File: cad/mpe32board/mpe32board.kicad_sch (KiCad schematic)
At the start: 2 parts, among them J1 Conn_ST_STDC14, U2 STM32H743VIHx

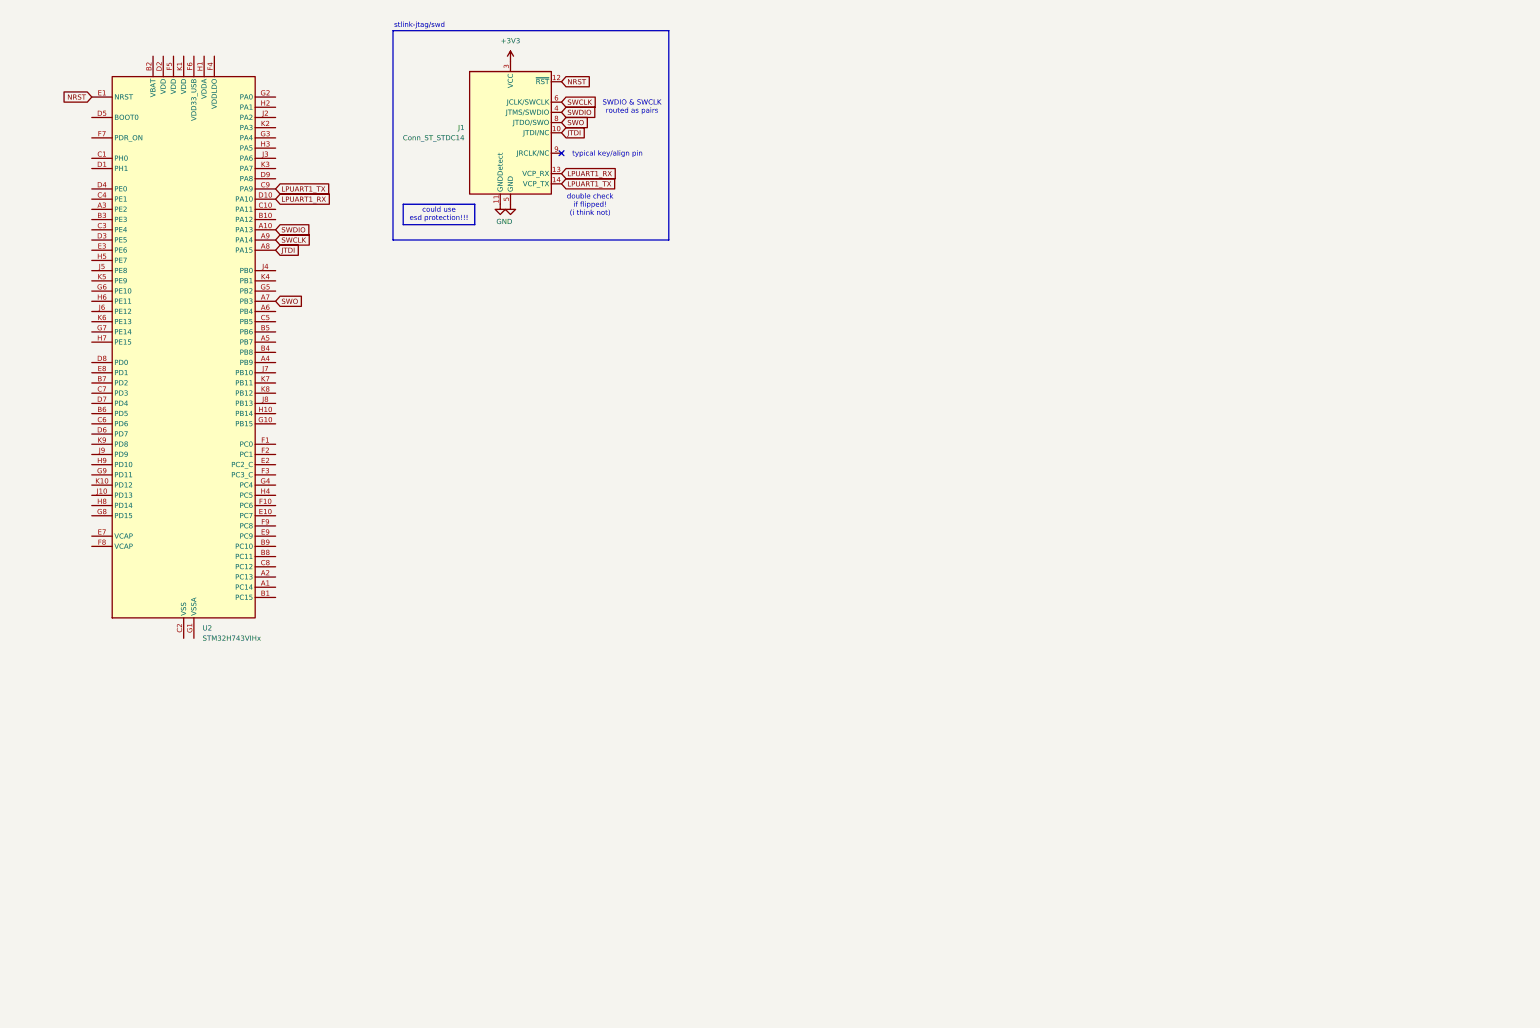
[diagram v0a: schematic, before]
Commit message: more pcb additions + research
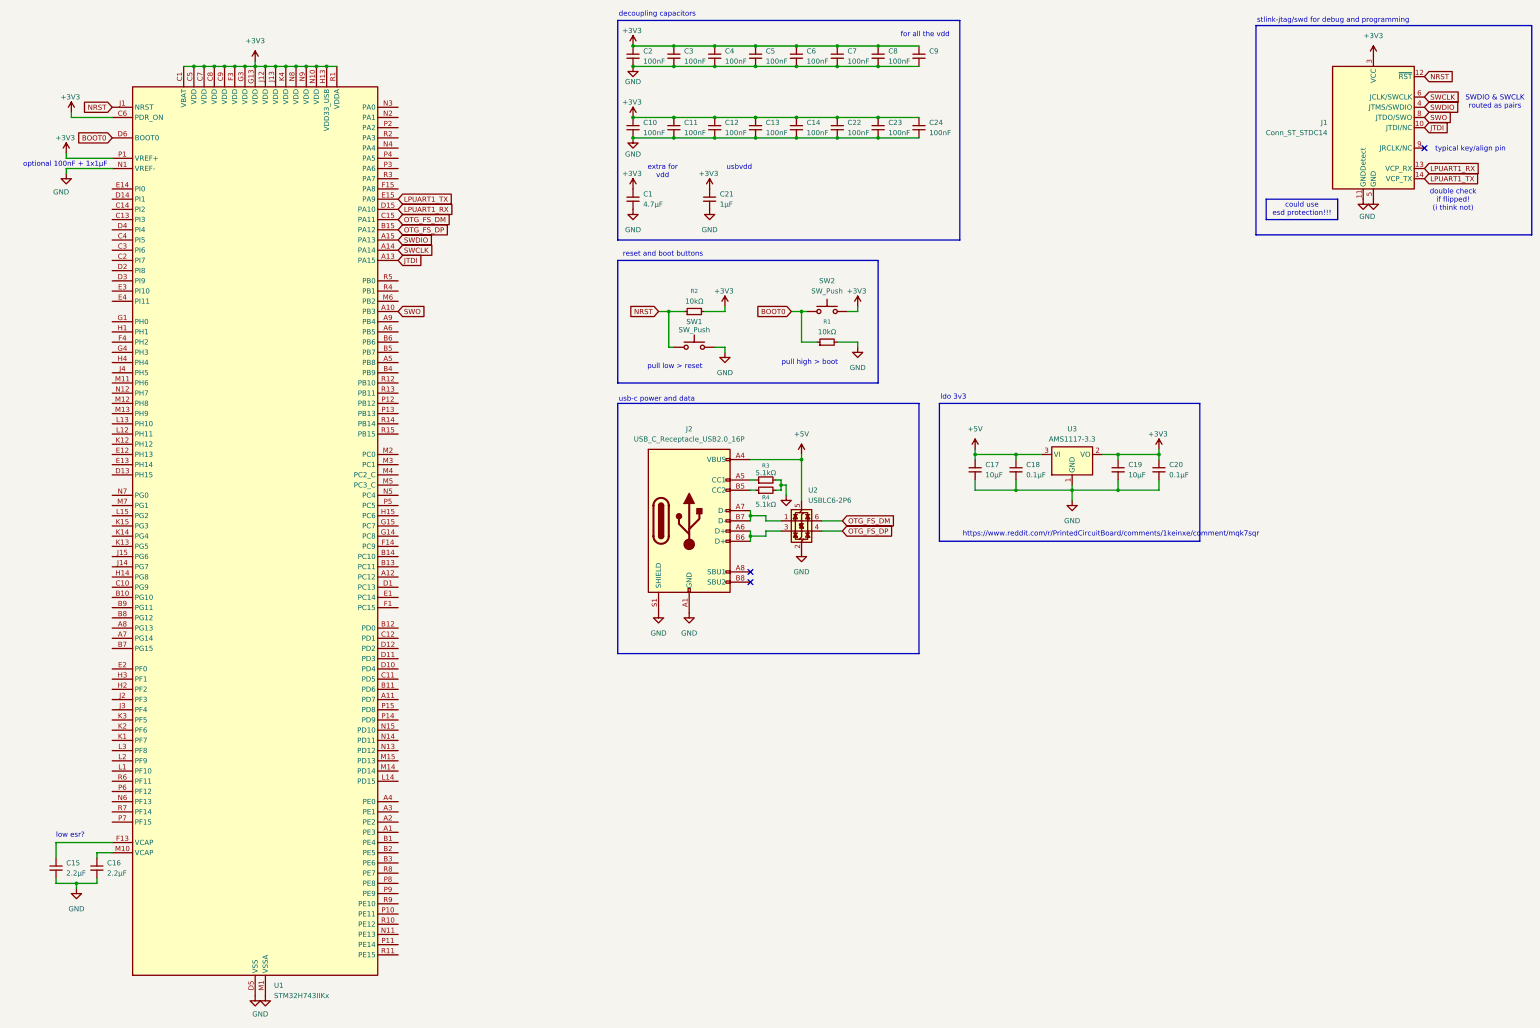
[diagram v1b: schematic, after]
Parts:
- removed U2: STM32H743VIHx, Package_BGA:TFBGA-100_8x8mm_Layout10x10_P0.8mm, symbol MCU_ST_STM32H7:STM32H743VIHx
- added C1: 4.7μF, symbol Device:C_Small
- added C10, C11, C12, C13, C14, C2, C22, C23, C24, C3, C4, C5, C6, C7, C8, C9: 100nF, symbol Device:C_Small
- added C15, C16: 2.2μF, symbol Device:C_Small
- added C17, C19: 10μF, symbol Device:C_Small
- added C18, C20: 0.1μF, symbol Device:C_Small
- added C21: 1μF, symbol Device:C_Small
- added J2: USB_C_Receptacle_USB2.0_16P, symbol Connector:USB_C_Receptacle_USB2.0_16P
- added R1, R2: 10kΩ, symbol Device:R_Small
- added R3, R4: 5.1kΩ, symbol Device:R_Small
- added SW1, SW2: SW_Push, symbol Switch:SW_Push
- added U1: STM32H743IIKx, Package_BGA:UFBGA-201_10x10mm_Layout15x15_P0.65mm, symbol MCU_ST_STM32H7:STM32H743IIKx
- added U2: USBLC6-2P6, Package_TO_SOT_SMD:SOT-666, symbol Power_Protection:USBLC6-2P6
- added U3: AMS1117-3.3, Package_TO_SOT_SMD:SOT-223-3_TabPin2, symbol Regulator_Linear:AMS1117-3.3
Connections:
- net +3V3: now also C1.1, C10.1, C11.1, C12.1, C13.1, C14.1, C19.1, C2.1, C20.1, C21.1, C22.1, C23.1, C24.1, C3.1, C4.1, C5.1, C6.1, C7.1, C8.1, C9.1, R2.2, SW2.2, U1.C1 (VBAT), U1.C5 (VDD), U1.C6 (PDR_ON), U1.C7 (VDD), U1.C8 (VDD), U1.C9 (VDD), U1.F3 (VDD), U1.G13 (VDD), U1.G3 (VDD), U1.H13 (VDD33_USB), U1.J12 (VDD), U1.J13 (VDD), U1.K4 (VDD), U1.N10 (VDD), U1.N8 (VDD), U1.N9 (VDD), U1.P1 (VREF+), U1.R1 (VDDA), U3.2 (VO)
- net GND: now also C1.2, C10.2, C11.2, C12.2, C13.2, C14.2, C15.2, C16.2, C17.2, C18.2, C19.2, C2.2, C20.2, C21.2, C22.2, C23.2, C24.2, C3.2, C4.2, C5.2, C6.2, C7.2, C8.2, C9.2, J2.A1 (GND), J2.A12 (GND), J2.B1 (GND), J2.B12 (GND), J2.S1 (SHIELD), R1.2, R3.2, R4.2, SW1.2, U1.D5 (VSS), U1.D7 (VSS), U1.D8 (VSS), U1.D9 (VSS), U1.F10 (VSS), U1.F12 (VSS), U1.F2 (VSS), U1.F6 (VSS), U1.F7 (VSS), U1.F8 (VSS), U1.F9 (VSS), U1.G10 (VSS), U1.G12 (VSS), U1.G2 (VSS), U1.G6 (VSS), U1.G7 (VSS), U1.G8 (VSS), U1.G9 (VSS), U1.H10 (VSS), U1.H12 (VSS), U1.H6 (VSS), U1.H7 (VSS), U1.H8 (VSS), U1.H9 (VSS), U1.J10 (VSS), U1.J6 (VSS), U1.J7 (VSS), U1.J8 (VSS), U1.J9 (VSS), U1.K10 (VSS), U1.K6 (VSS), U1.K7 (VSS), U1.K8 (VSS), U1.K9 (VSS), U1.L4 (VSS), U1.M1 (VSSA), U1.M8 (VSS), U1.M9 (VSS), U1.N1 (VREF-), U2.2 (GND), U3.1 (GND)
- net JTDI: now also U1.A13 (PA15)
- net LPUART1_RX: now also U1.D15 (PA10)
- net LPUART1_TX: now also U1.E15 (PA9)
- net NRST: now also R2.1, SW1.1, U1.J1 (NRST)
- net SWCLK: now also U1.A14 (PA14)
- net SWDIO: now also U1.A15 (PA13)
- net SWO: now also U1.A10 (PB3)
- new net: C16.1, U1.M10 (VCAP)
- new net: J2.B5 (CC2), R4.1
- new net: J2.A7 (D-), J2.B7 (D-), U2.1 (I/O1)
- new net: J2.A6 (D+), J2.B6 (D+), U2.3 (I/O2)
- new net: J2.A5 (CC1), R3.1
- new net: C15.1, U1.F13 (VCAP)
- new net +5V: C17.1, C18.1, J2.A4 (VBUS), J2.A9 (VBUS), J2.B4 (VBUS), J2.B9 (VBUS), U2.5 (VBUS), U3.3 (VI)
- new net BOOT0: R1.1, SW2.1, U1.D6 (BOOT0)
- new net OTG_FS_DM: U1.C15 (PA11), U2.6 (I/O1)
- new net OTG_FS_DP: U1.B15 (PA12), U2.4 (I/O2)
- no-connect marks 1 -> 3
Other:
- note added: "decoupling capacitors"
- note added: "extra for vdd"
- note added: "for all the vdd"
- note added: "https://www.reddit.com/r/PrintedCircuitBoard/comments/1keinxe/comment/mqk7sqr"
- note added: "ldo 3v3"
- note added: "low esr?"
- note added: "optional 100nF + 1x1μF"
- note added: "pull high > boot"
- note added: "pull low > reset"
- note added: "reset and boot buttons"
- note added: "stlink-jtag/swd for debug and programming"
- note added: "usb-c power and data"
- note added: "usbvdd"
- note removed: "stlink-jtag/swd"
- moved on the sheet: J1
